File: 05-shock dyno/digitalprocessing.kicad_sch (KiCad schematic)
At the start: 9 parts, among them U1 INA827AIDGK, U2 AD5626BRMZ

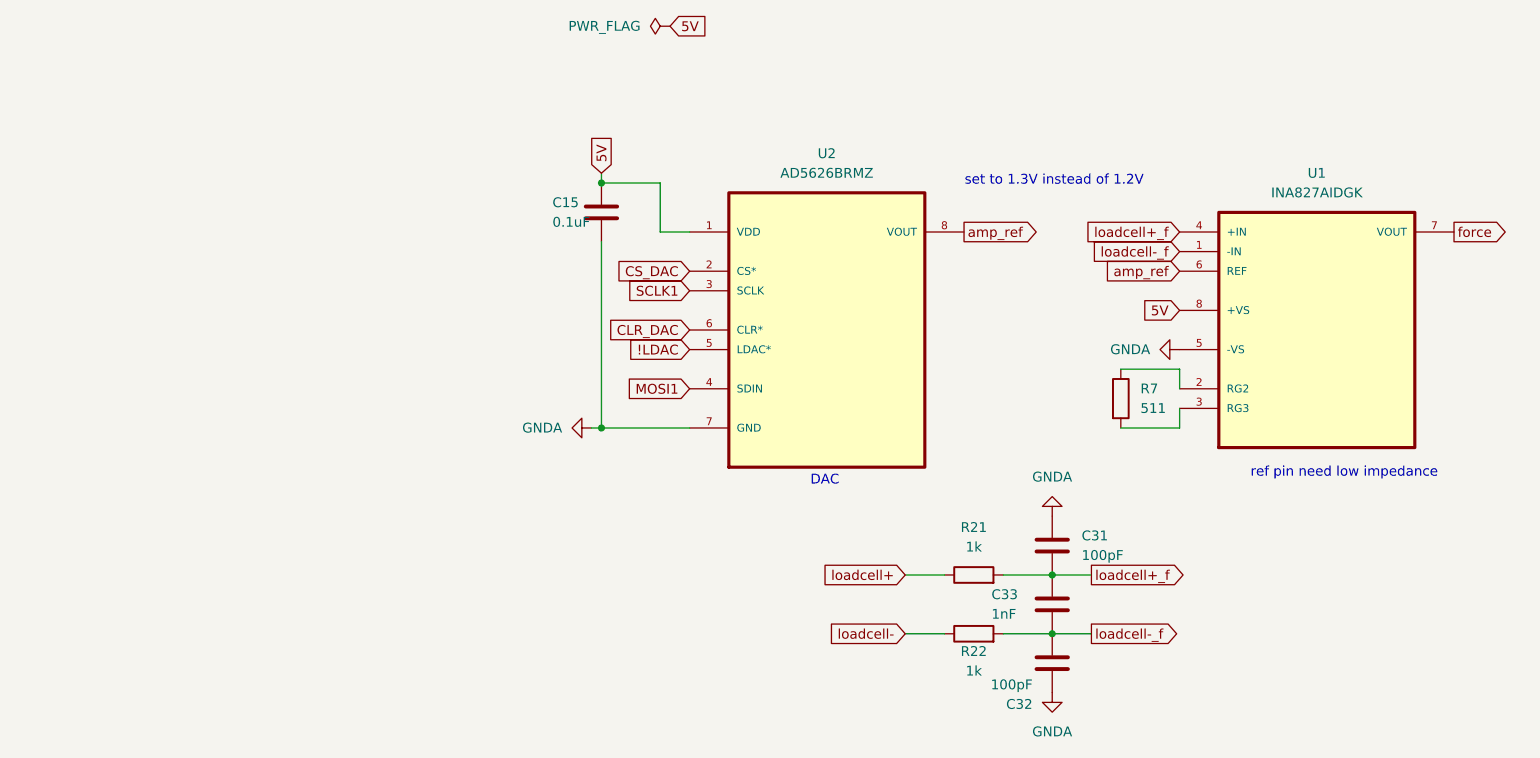
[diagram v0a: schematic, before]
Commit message: layout updates
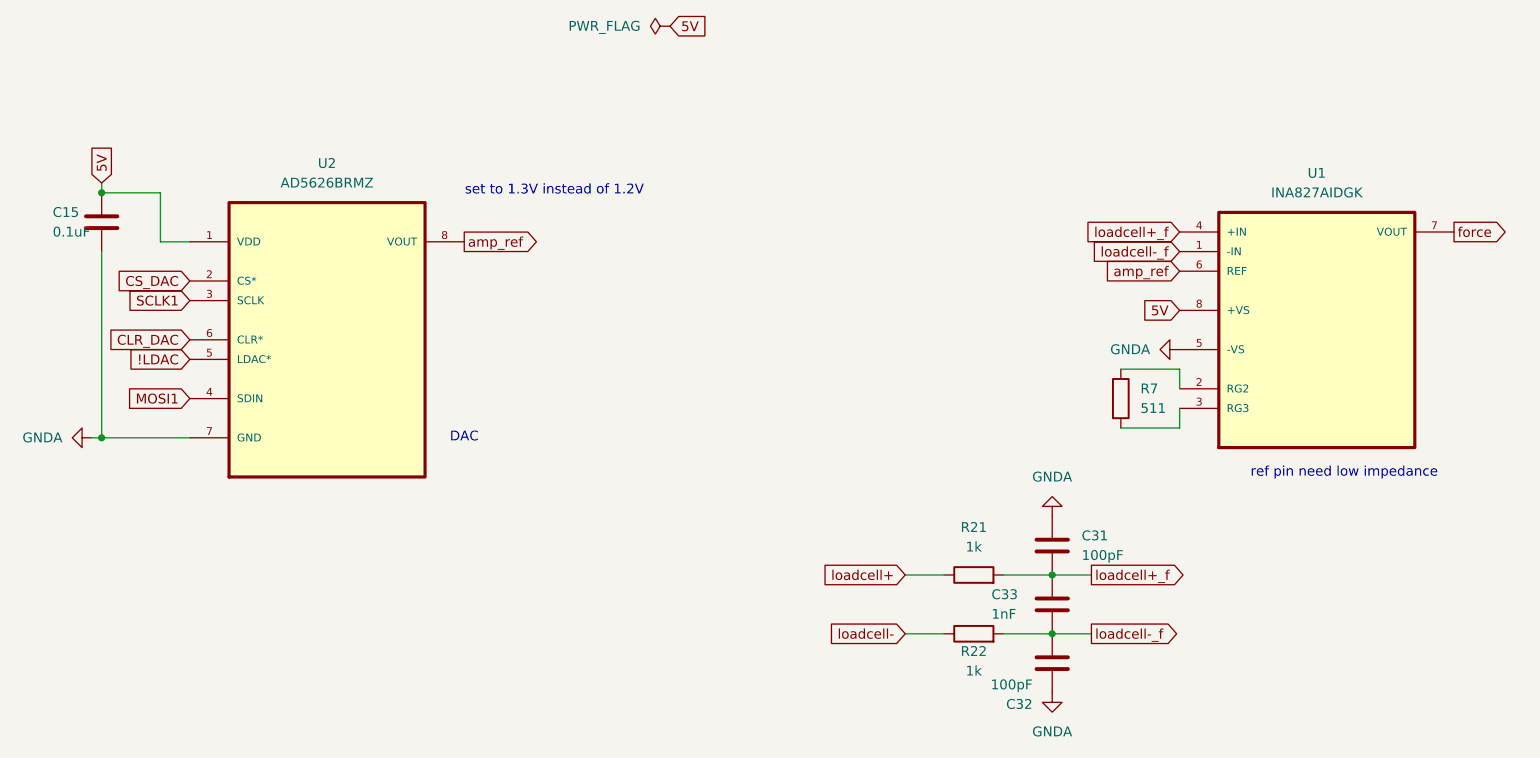
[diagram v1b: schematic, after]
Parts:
- C15: footprint (none) -> Capacitor_SMD:C_0402_1005Metric
- C31, C32, C33, R21, R22: footprint (none) -> Capacitor_SMD:C_0603_1608Metric
- R7: footprint (none) -> Capacitor_SMD:C_0805_2012Metric
- U1: footprint INA827AIDGK:SOP65P490X110-8N -> 00-footprints:INA827AIDGK
- U2: footprint AD5626BRMZ:SOP65P490X110-8N -> 00-footprints:AD5626BRMZ
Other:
- moved on the sheet: C15, U2
